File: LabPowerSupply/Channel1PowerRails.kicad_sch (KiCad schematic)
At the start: 8 parts

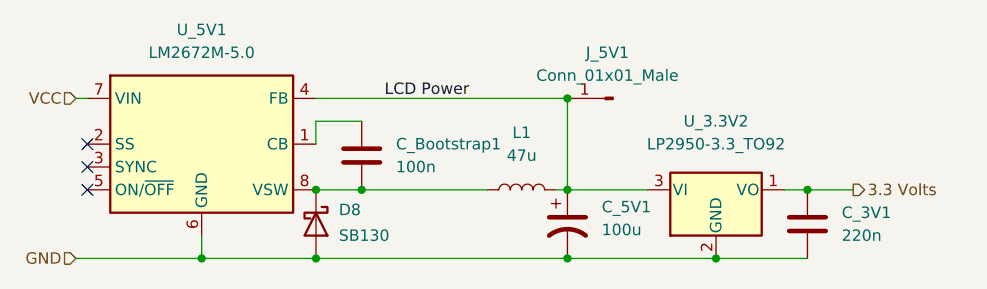
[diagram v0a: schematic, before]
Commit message: more work
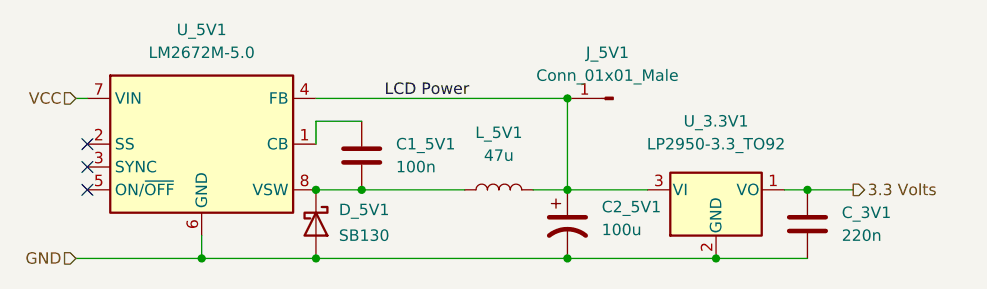
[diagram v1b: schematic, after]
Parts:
- renumbered C_Bootstrap1 to C1_5V1, C_5V1 to C2_5V1, D8 to D_5V1, L1 to L_5V1, U_3.3V2 to U_3.3V1
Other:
- moved on the sheet: L_5V1
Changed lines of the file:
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@@
     (stroke (width 0) (type default) (color 0 0 0 0))
   )
-  (wire (pts (xy 158.75 99.06) (xy 144.78 99.06))
+  (wire (pts (xy 156.21 99.06) (xy 144.78 99.06))
     (stroke (width 0) (type default) (color 0 0 0 0))
   )
@@
     (stroke (width 0) (type default) (color 0 0 0 0))
   )
-  (wire (pts (xy 166.37 99.06) (xy 167.64 99.06))
+  (wire (pts (xy 163.83 99.06) (xy 167.64 99.06))
     (stroke (width 0) (type default) (color 0 0 0 0))
   )
@@
   (symbol (lib_id "Regulator_Linear:LP2950-3.3_TO92") (at 184.15 99.06 0) (unit 1)
     (in_bom yes) (on_board yes) (fields_autoplaced)
-    (property "Reference" "U_3.3V2" (id 0) (at 184.15 91.44 0))
+    (property "Reference" "U_3.3V1" (id 0) (at 184.15 91.44 0))
     (property "Value" "LP2950-3.3_TO92" (id 1) (at 184.15 93.98 0))
     (property "Footprint" "Package_TO_SOT_THT:TO-92_Inline" (id 2) (at 184.15 93.345 0)
@@
   (symbol (lib_id "Device:C_Polarized_US") (at 167.64 102.87 0) (unit 1)
     (in_bom yes) (on_board yes) (fields_autoplaced)
-    (property "Reference" "C_5V1" (id 0) (at 171.45 100.9649 0)
+    (property "Reference" "C2_5V1" (id 0) (at 171.45 100.9649 0)
       (effects (font (size 1.27 1.27)) (justify left))
     )
@@
   (symbol (lib_id "Diode:SB130") (at 139.7 102.87 270) (unit 1)
     (in_bom yes) (on_board yes)
-    (property "Reference" "D8" (id 0) (at 142.24 101.2824 90)
+    (property "Reference" "D_5V1" (id 0) (at 142.24 101.2824 90)
       (effects (font (size 1.27 1.27)) (justify left))
     )
@@
     (pin "2")
   )
-  (symbol (lib_id "Device:L") (at 162.56 99.06 90) (unit 1)
+  (symbol (lib_id "Device:L") (at 160.02 99.06 90) (unit 1)
     (in_bom yes) (on_board yes) (fields_autoplaced)
-    (property "Reference" "L1" (id 0) (at 162.56 92.71 90))
-    (property "Value" "47u" (id 1) (at 162.56 95.25 90))
-    (property "Footprint" "Inductor_THT:L_Radial_D6.0mm_P4.00mm" (id 2) (at 162.56 99.06 0)
+    (property "Reference" "L_5V1" (id 0) (at 160.02 92.71 90))
+    (property "Value" "47u" (id 1) (at 160.02 95.25 90))
+    (property "Footprint" "Inductor_THT:L_Radial_D6.0mm_P4.00mm" (id 2) (at 160.02 99.06 0)
       (effects (font (size 1.27 1.27)) hide)
     )
-    (property "Datasheet" "~" (id 3) (at 162.56 99.06 0)
+    (property "Datasheet" "~" (id 3) (at 160.02 99.06 0)
       (effects (font (size 1.27 1.27)) hide)
     )
@@
   (symbol (lib_id "Device:C") (at 144.78 95.25 0) (unit 1)
     (in_bom yes) (on_board yes) (fields_autoplaced)
-    (property "Reference" "C_Bootstrap1" (id 0) (at 148.59 93.9799 0)
+    (property "Reference" "C1_5V1" (id 0) (at 148.59 93.9799 0)
       (effects (font (size 1.27 1.27)) (justify left))
     )
